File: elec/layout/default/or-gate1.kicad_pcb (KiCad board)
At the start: 2 copper layers, 225.7 x 100.8 mm, 0 parts

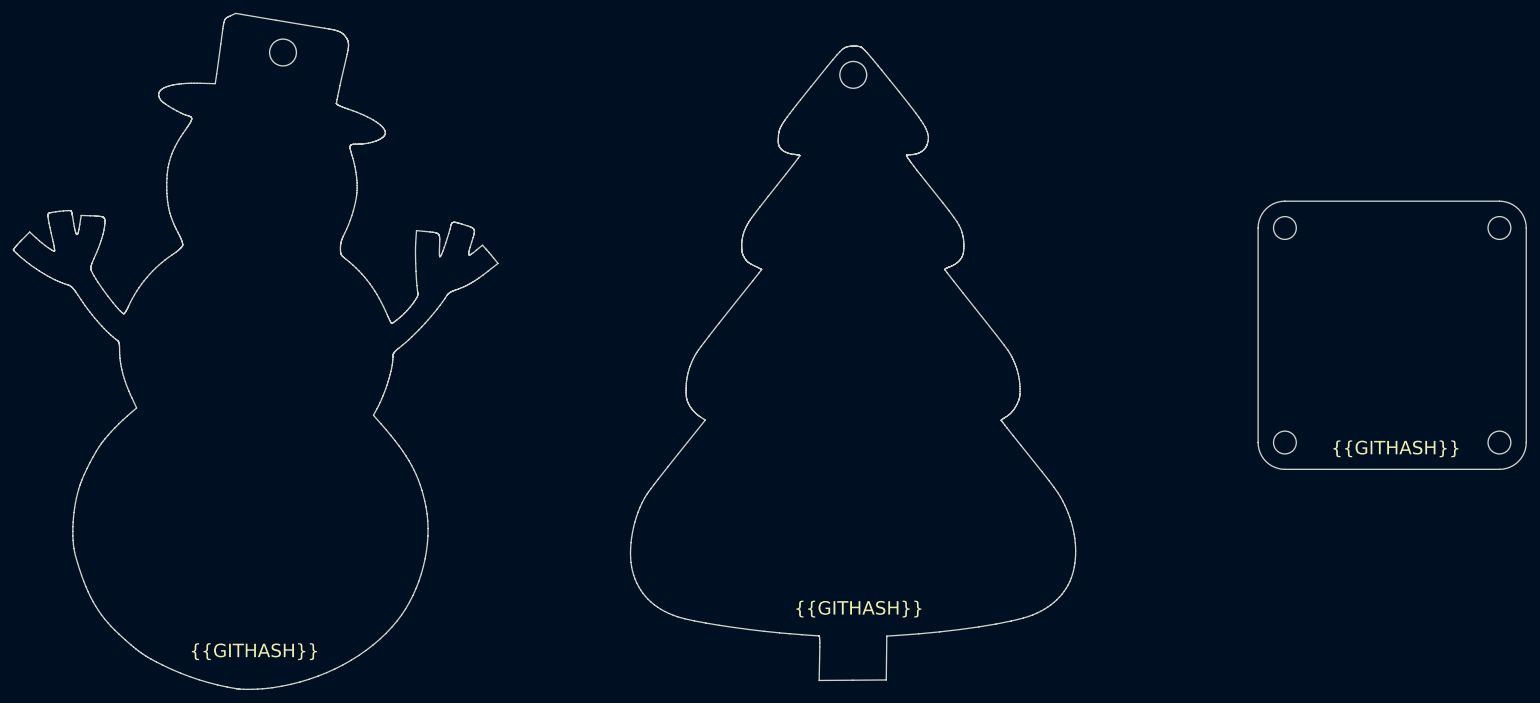
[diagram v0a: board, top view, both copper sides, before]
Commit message: Update layout
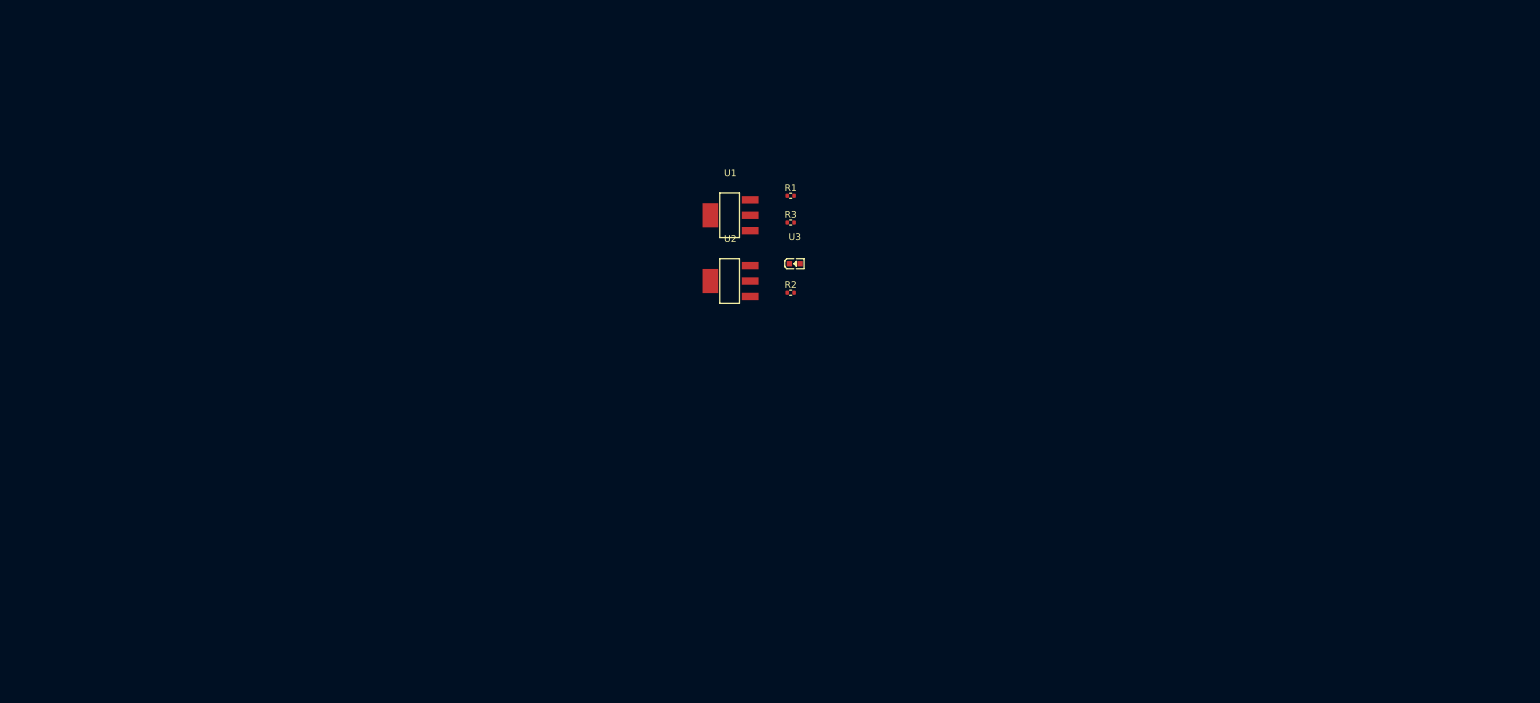
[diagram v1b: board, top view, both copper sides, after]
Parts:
- added R1: 10.0 +/- 1.0 kiloohm, footprints:R0402, F.Cu at (151.9, 77.0)
- added R2: 1.0 +/- 0.10000000000000003 kiloohm, footprints:R0402, F.Cu at (151.9, 91.4)
- added R3: 1.0 +/- 0.10000000000000003 kiloohm, footprints:R0402, F.Cu at (151.9, 81.0)
- added U1: , footprints1:SOT-223-3_L6.5-W3.4-P2.30-LS7.0-BR, F.Cu at (142.9, 79.9)
- added U2: , footprints1:SOT-223-3_L6.5-W3.4-P2.30-LS7.0-BR, F.Cu at (142.9, 89.7)
- added U3: , footprints:LED0603-RD, F.Cu at (152.5, 87.1)
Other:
- board outline removed
- board text removed: "{{GITHASH}}"
